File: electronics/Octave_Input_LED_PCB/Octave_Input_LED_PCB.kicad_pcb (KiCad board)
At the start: 2 copper layers, 76.2 x 57.2 mm, 37 parts, among them J3 Conn_01x12, SW1 SW_Hot_Swap_Socket, SW10 SW_Hot_Swap_Socket, SW11 SW_Hot_Swap_Socket, SW12 SW_Hot_Swap_Socket, SW2 SW_Hot_Swap_Socket, SW3 SW_Hot_Swap_Socket, SW4 SW_Hot_Swap_Socket, SW5 SW_Hot_Swap_Socket, SW6 SW_Hot_Swap_Socket, SW7 SW_Hot_Swap_Socket, SW8 SW_Hot_Swap_Socket, SW9 SW_Hot_Swap_Socket

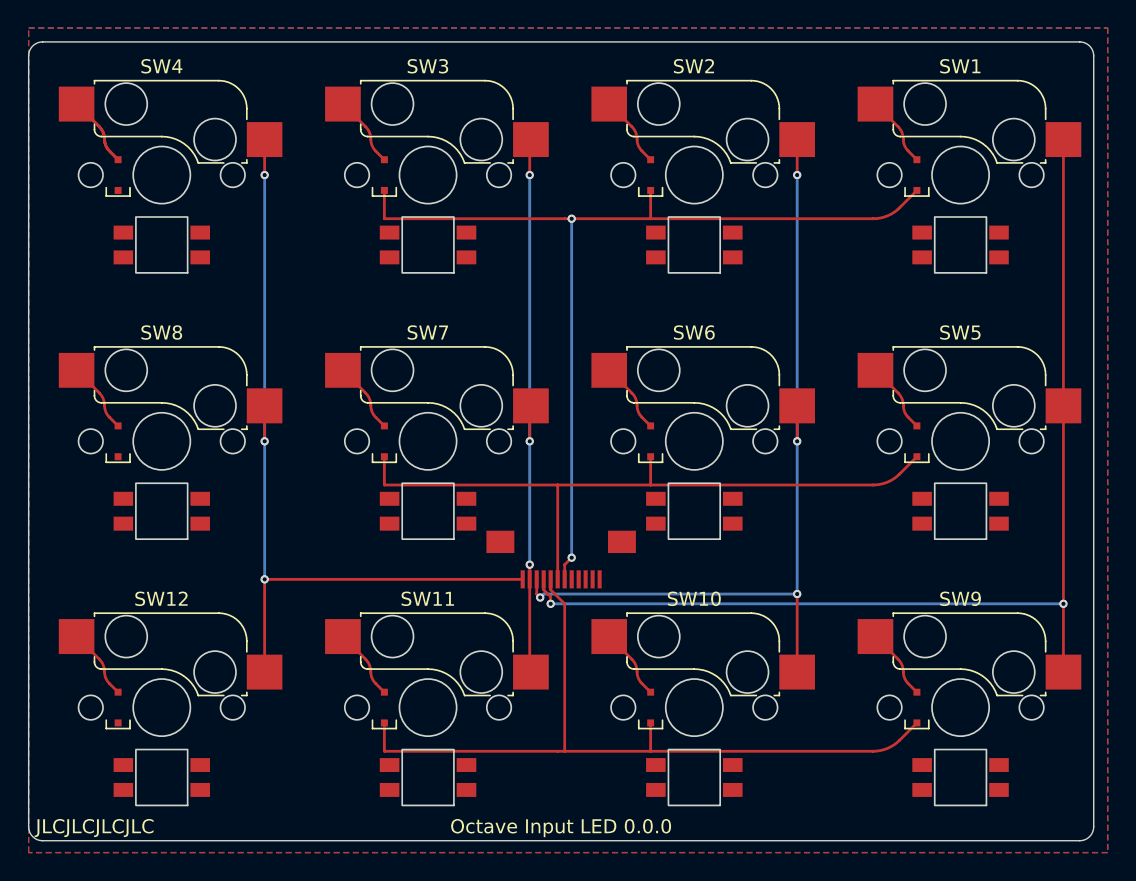
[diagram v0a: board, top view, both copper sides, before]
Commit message: Route PCB
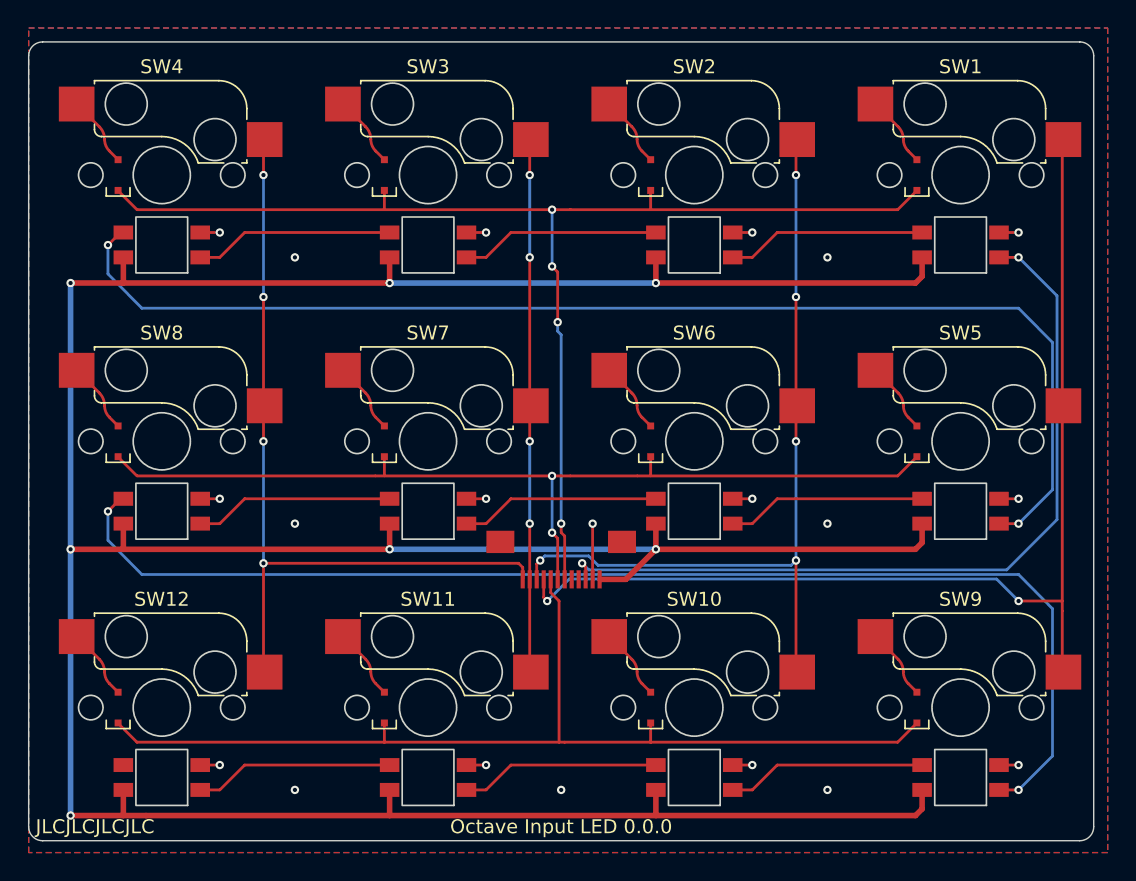
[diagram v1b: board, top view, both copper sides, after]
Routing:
- net +3V3: track 0.00 -> 246.9 mm, vias 0 -> 7
- net Net-(LED204-Pad2): track 0.00 -> 88.5 mm, vias 0 -> 2
- net Net-(LED208-Pad2): track 0.00 -> 88.3 mm, vias 0 -> 2
- net IO0_MPU: track 0.00 -> 58.2 mm, vias 0 -> 2
- net GND: track 0.00 -> 20.8 mm, vias 0 -> 20
- net ROW0_UI: track 68.9 -> 87.8 mm, vias 2 -> 4
- net ROW1_UI: track 49.6 -> 68.6 mm, vias 0 -> 2
- net ROW2_UI: track 55.6 -> 72.9 mm
- net Net-(LED209-Pad2): track 0.00 -> 14.3 mm
- net Net-(LED205-Pad2): track 0.00 -> 14.3 mm
- net Net-(LED201-Pad2): track 0.00 -> 14.3 mm
- net Net-(LED211-Pad2): track 0.00 -> 14.3 mm
- net Net-(LED210-Pad2): track 0.00 -> 14.3 mm
- net Net-(LED207-Pad2): track 0.00 -> 14.3 mm
- net Net-(LED206-Pad2): track 0.00 -> 14.3 mm
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- added copper zone on B.Cu, net GND
- added copper zone on F.Cu, net GND
- removed copper zone on B.Cu, net (none)
- removed copper zone on F.Cu, net (none)
